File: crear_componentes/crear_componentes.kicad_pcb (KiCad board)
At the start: 2 copper layers, 5 parts, among them J1 Conn_01x02_Female, SW1 SW_Push, U1 ULN2003A

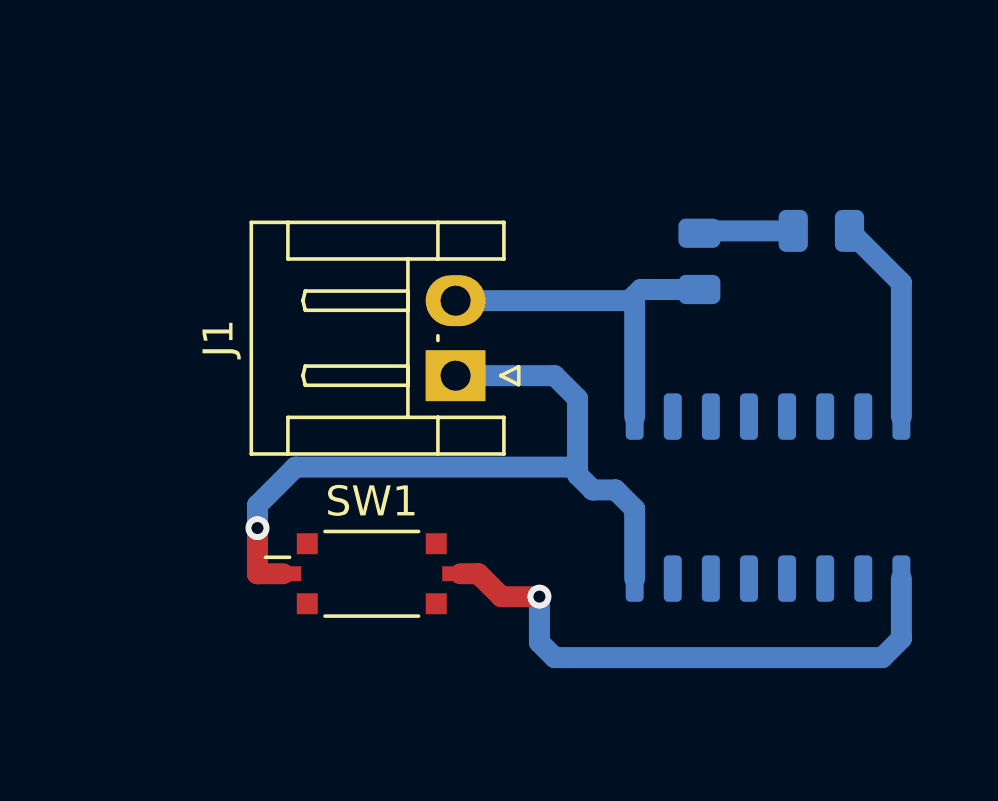
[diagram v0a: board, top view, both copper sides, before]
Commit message: Hemos trabajado en nueva version de sistema de medicio
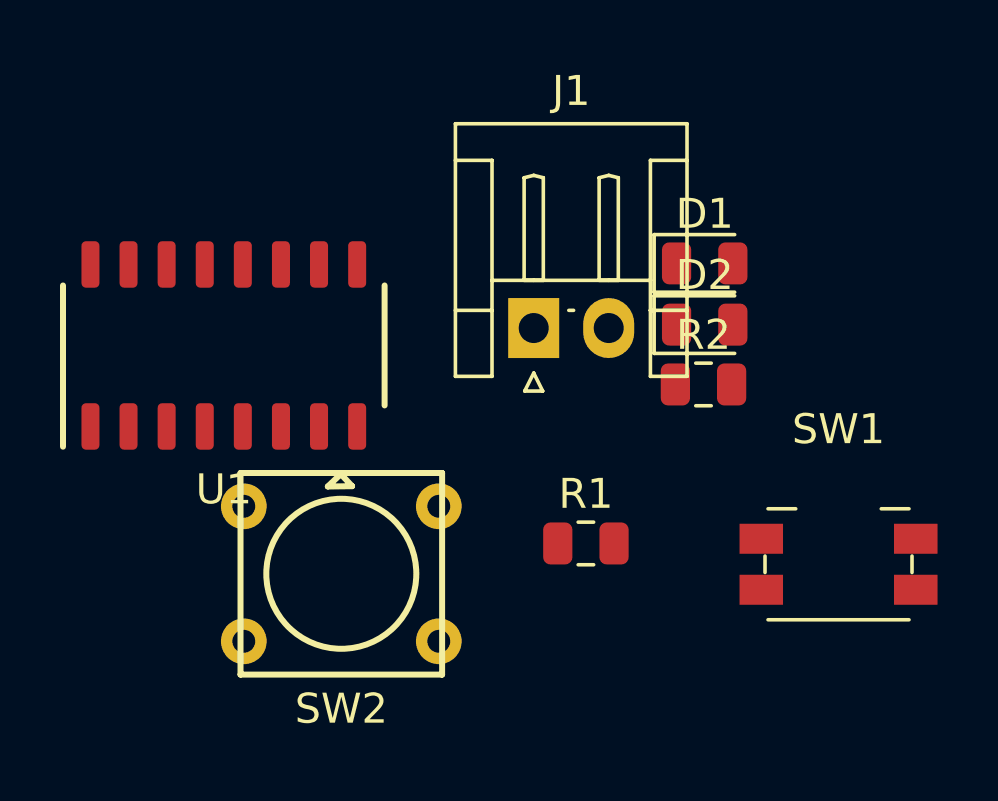
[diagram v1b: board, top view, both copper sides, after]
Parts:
- added D2: LED, LED_SMD:LED_0805_2012Metric, F.Cu at (147.2, 89.7)
- added R2: R, Resistor_SMD:R_0805_2012Metric, F.Cu at (147.2, 91.7)
- added SW2: TopPush, Mi_breria:TopPush, F.Cu at (135.1, 98.0)
- D1, R1, U1: moved to F.Cu
- SW1: footprint Button_Switch_SMD:SW_DIP_SPSTx01_Slide_Copal_CVS-01xB_W5.9mm_P1mm -> Button_Switch_SMD:Panasonic_EVQPUK_EVQPUB
- moved U1 18.8 mm to (131.2, 90.4), turned to 0 degrees
- moved SW1 15.6 mm to (151.7, 97.7)
- moved R1 10.1 mm to (143.3, 97.0), turned to 0 degrees
- moved D1 4.04 mm to (147.2, 87.7), turned to 0 degrees
- moved J1 3.05 mm to (141.5, 89.9), turned to 0 degrees
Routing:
- net +5V: track 26.0 -> 0.00 mm, vias 1 -> 0
- net Net-(SW1-Pad2): track 19.0 -> 0.00 mm, vias 1 -> 0
- net GND: track 12.3 -> 0.00 mm
- net Net-(D1-Pad1): track 6.91 -> 0.00 mm
- net Net-(D1-Pad2): track 3.16 -> 0.00 mm
